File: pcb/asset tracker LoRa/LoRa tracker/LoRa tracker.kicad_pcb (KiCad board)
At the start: 2 copper layers, 100 x 100 mm, 57 parts, among them CON1 jtag, CON2 jtag, J1 Screw_Terminal_01x02, J2 Screw_Terminal_01x02, Q1 BSS138, U1 INA219BxDCN, U2 R-783.3-1.0, U3 LIS3DH, U4 G3VM-61HR2(TR05), U5 DS28CM00R-A00+T, U6 nRF52810-QFxx, U7 ATSAMD21, Y1 326MhZ

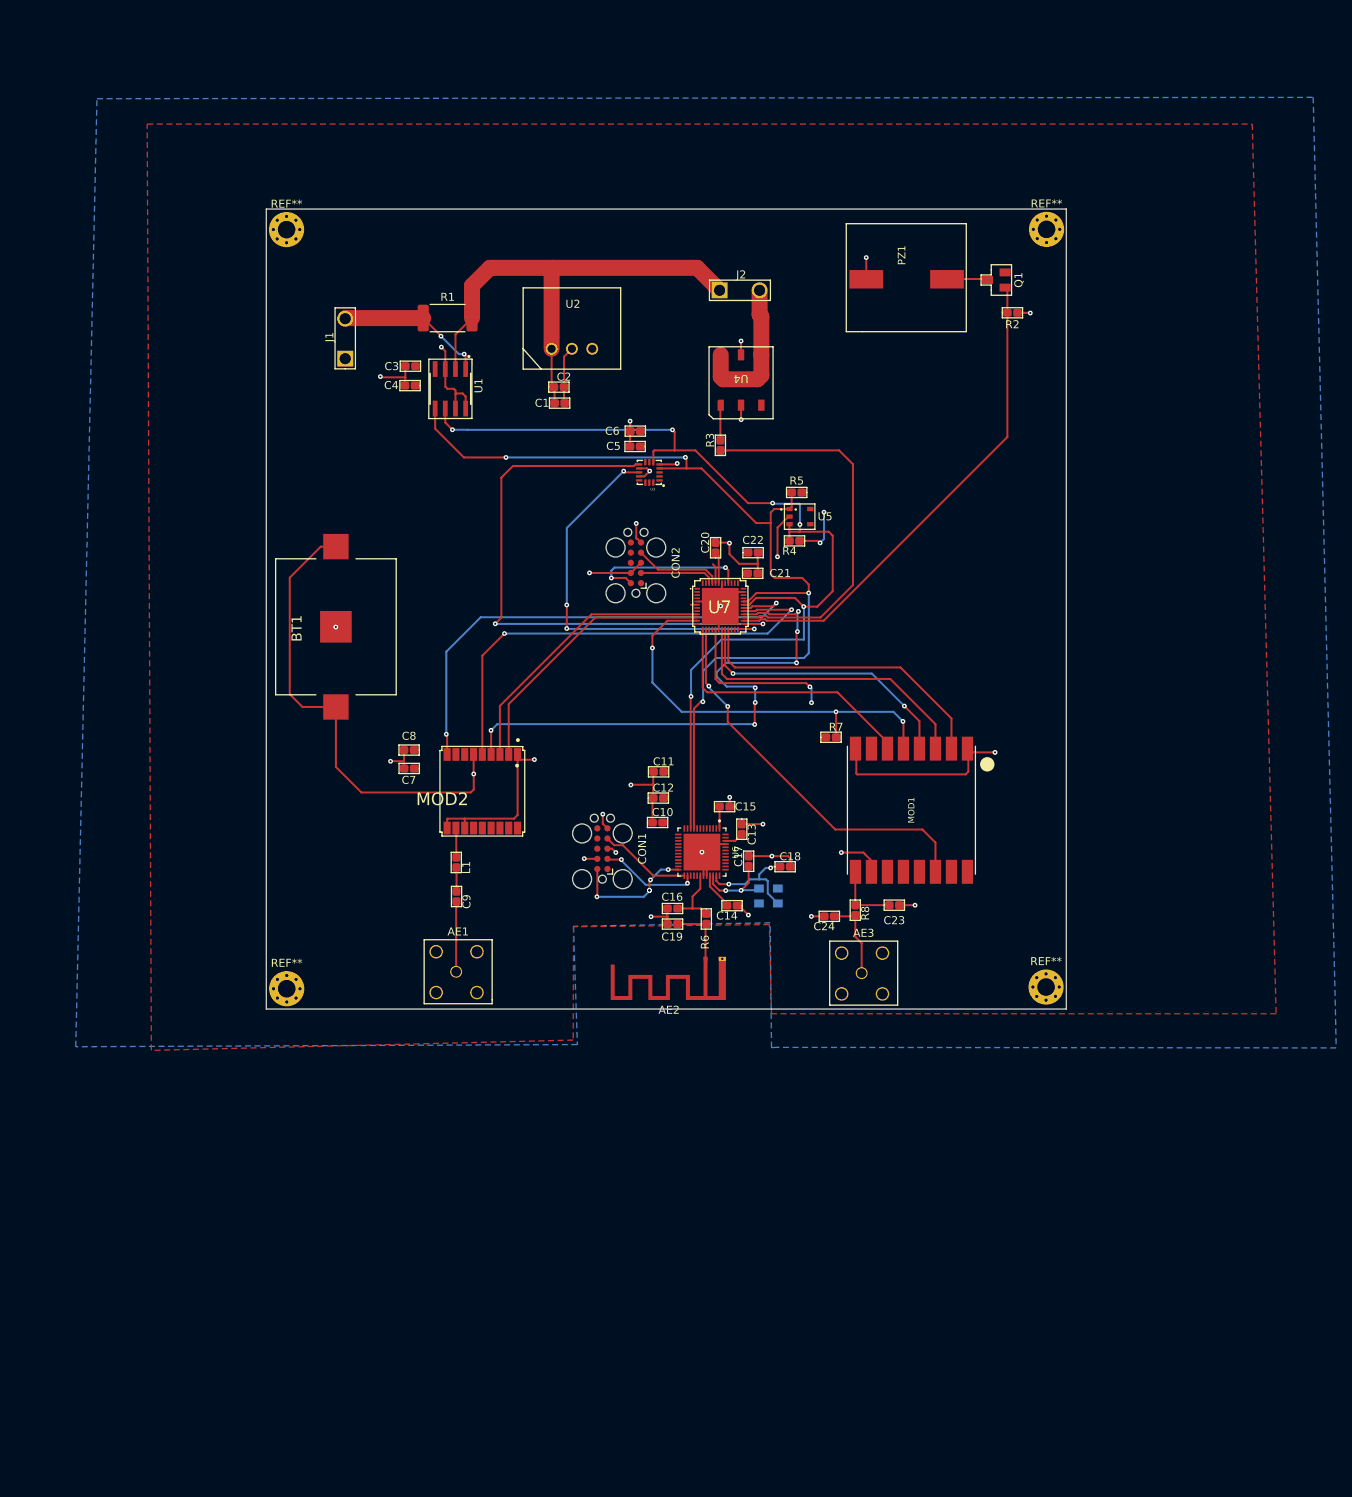
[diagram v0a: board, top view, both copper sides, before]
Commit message: pcb kastje
pcb in kastje getekend
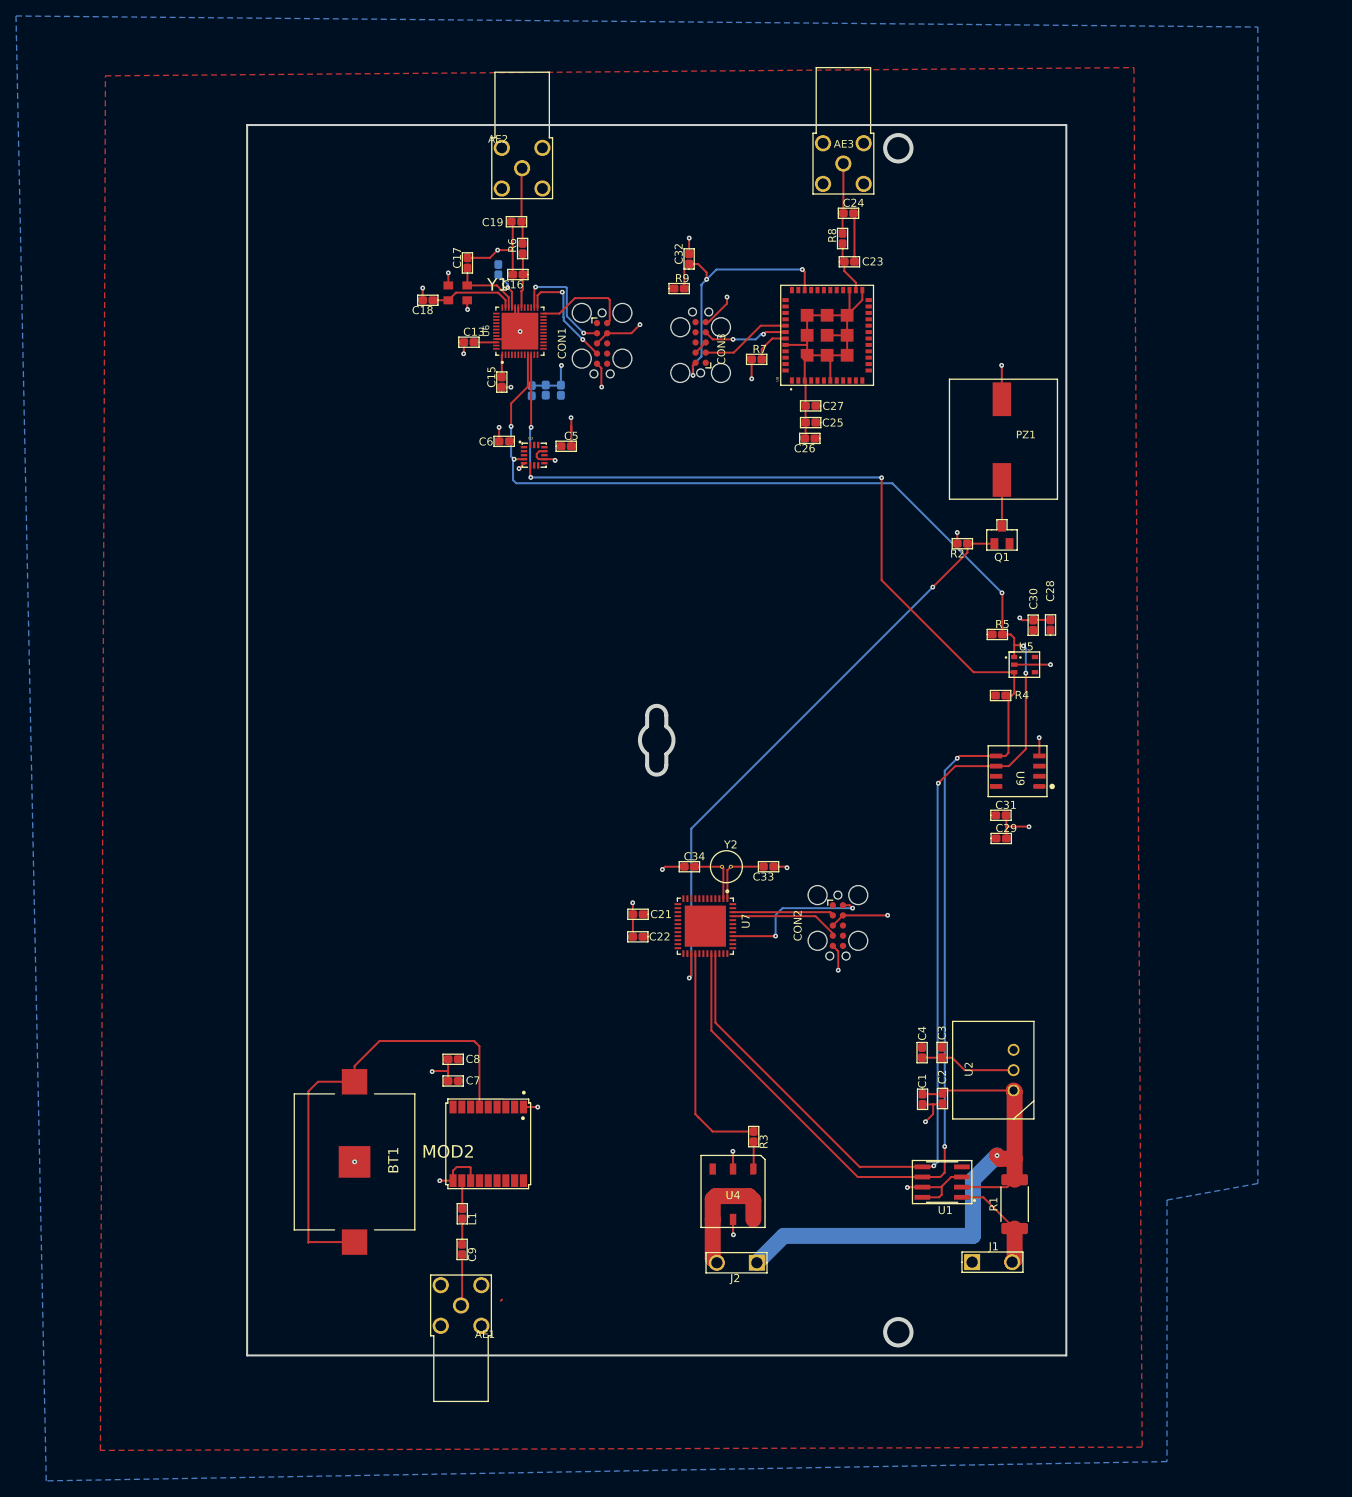
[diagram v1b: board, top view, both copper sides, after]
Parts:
- removed C20: 10uF, vanalles:0603
- removed MOD1: rfm95, Module:RFM69HW
- removed REF** (x4): MountingHole_2.2mm_M2_Pad_Via, vanalles:MountingHole_2.2mm_M2_Pad_Via
- added C25: 10uF, vanalles:0603, F.Cu at (130.2, 64.6)
- added C26: 1uF, vanalles:0603, F.Cu at (130.1, 66.5)
- added C27: 0.1uF, vanalles:0603, F.Cu at (130.2, 62.5)
- added C28: 100nF, vanalles:0603, F.Cu at (160.2, 89.8)
- added C29: 10uF, vanalles:0603, F.Cu at (154.1, 116.5)
- added C30: 100nF, vanalles:0603, F.Cu at (158.0, 89.9)
- added C31: 10uF, vanalles:0603, F.Cu at (154.0, 113.6)
- added C32: 100nF, vanalles:0603, F.Cu at (115.0, 44.1)
- added C33: 20pF, vanalles:0603, F.Cu at (125.0, 120.1)
- added C34: 20pF, vanalles:0603, F.Cu at (115.1, 120.1)
- added CON3: jtag, connectors_user:Tag-Connect_TC2050-IDC-FP_2x05_P1.27mm_Vertical, F.Cu at (116.5, 54.5)
- added R9: 10K, vanalles:0603RL, F.Cu at (113.8, 47.8)
- added U8: murattaLora, Module:XCVR_CMWX1ZZABZ-078, F.Cu at (132.3, 53.6)
- added U9: ATECC608B, halfgeleiders:soic p1.27 lengt 5.40, F.Cu at (158.8, 110.0)
- added Y2: Crystal, vanalles:crystal tht, F.Cu at (119.2, 120.1)
- AE1, AE3: footprint connectors_user:sma_right angeld -> connectors_user:sma juist
- AE2: value Antenna -> Antenna_Shield; footprint vanalles:Texas_SWRA117D_2.4GHz_Right -> connectors_user:sma juist
- C10, C11, C12, C14: moved to B.Cu
- R7: footprint vanalles:0603 -> vanalles:0603RL
- U7: value ATSAMD21 -> ATSAMD21G18A-M; footprint halfgeleiders:QFN49P40_600X600X90L40X20T460N -> halfgeleiders:QFN50P700X700X90-49N
- Y1: moved to F.Cu
- moved J1 141.0 mm to (153.0, 169.5), turned to 0 degrees
- moved R1 131.5 mm to (155.7, 162.2), turned to 90 degrees
- moved J2 121.5 mm to (121.0, 169.6), turned to 180 degrees
- moved U1 116.7 mm to (146.7, 159.5), turned to 180 degrees
- moved C3 108.5 mm to (146.7, 143.3), turned to -90 degrees
- moved U4 108.1 mm to (120.5, 164.2), turned to 0 degrees
- moved U2 105.7 mm to (155.6, 145.5), turned to 90 degrees
- moved AE2 105.6 mm to (94.2, 28.5)
- moved AE3 105.4 mm to (134.3, 28.0), turned to 180 degrees
- moved C4 105.1 mm to (144.2, 143.3), turned to -90 degrees
- moved C2 101.0 mm to (146.7, 149.0), turned to -90 degrees
- moved C1 98.1 mm to (144.2, 149.1), turned to -90 degrees
- moved C19 89.9 mm to (93.5, 39.4)
- moved C24 87.9 mm to (135.0, 38.4), turned to 0 degrees
- moved R6 86.9 mm to (94.2, 42.8), turned to 90 degrees
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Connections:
- net /LoRa_RFM/ANT_RFM renamed /LoRa_RFM/ANT
- AE2 pad 1: Net-(AE2-Pad1) -> (no net)
- AE2 pad 2: (no net) -> GND
- AE3 pad 1: unconnected-(AE3-Pad1) -> Net-(AE3-Pad1)
- C19 pad 1: Net-(AE2-Pad1) -> (no net)
- C24 pad 1: Net-(C24-Pad1) -> Net-(AE3-Pad1)
- R6 pad 2: Net-(AE2-Pad1) -> (no net)
- R7 pad 1: +3V3 -> GND
- R7 pad 2: /CS -> Net-(R7-Pad2)
- R8 pad 2: Net-(C24-Pad1) -> Net-(AE3-Pad1)
- U7 pad 1: unconnected-(U7-Pad1) -> Net-(C33-Pad2)
- U7 pad 10: /TX -> /RX
- U7 pad 11: /CS -> /TX
- U7 pad 13: /RESET -> unconnected-(U7-Pad13)
- U7 pad 14: /IRQ -> unconnected-(U7-Pad14)
- U7 pad 19: /MOSI -> unconnected-(U7-Pad19)
- U7 pad 2: unconnected-(U7-Pad2) -> Net-(C34-Pad2)
- U7 pad 20: /SCK -> unconnected-(U7-Pad20)
- U7 pad 21: /MISO -> /MOSI
- U7 pad 22: unconnected-(U7-Pad22) -> /SCK
- U7 pad 23: unconnected-(U7-Pad23) -> /CS
- U7 pad 24: /INT1 -> /MISO
- U7 pad 25: /INT2 -> /INT1
- U7 pad 26: /BUZZER -> /INT2
- U7 pad 27: /SSR -> /BUZZER
- U7 pad 28: /PPS -> /SSR
- U7 pad 29: /WAKE -> /PPS
- U7 pad 30: /RESET_GPS -> /WAKE
- U7 pad 31: /SDA -> /RESET_GPS
- U7 pad 32: /SCL -> /SDA
- U7 pad 33: unconnected-(U7-Pad33) -> /SCL
- U7 pad 39: unconnected-(U7-Pad39) -> /RESET
- U7 pad 43: Net-(C20-Pad1) -> +3V3
- U7 pad 49: GND -> unconnected-(U7-Pad49)
- U7 pad 9: /RX -> unconnected-(U7-Pad9)
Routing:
- net /SCL: track 122.8 -> 212.7 mm, vias 4 -> 7
- net /SDA: track 126.2 -> 211.8 mm, vias 6 -> 5
- net /INT2: track 72.4 -> 0.00 mm, vias 2 -> 0
- net /PPS: track 71.0 -> 0.00 mm, vias 7 -> 0
- net /RESET_GPS: track 61.0 -> 0.00 mm, vias 2 -> 0
- net /WAKE: track 59.5 -> 0.00 mm, vias 2 -> 0
- net /CS: track 52.2 -> 0.00 mm, vias 3 -> 0
- net /INT1: track 50.2 -> 0.00 mm, vias 4 -> 0
- net /IRQ: track 48.6 -> 0.00 mm, vias 2 -> 0
- net /MISO: track 38.6 -> 0.00 mm
- net /MOSI: track 37.9 -> 0.00 mm
- net /RX: track 35.5 -> 0.00 mm
- net /SCK: track 35.1 -> 0.00 mm, vias 2 -> 0
- net /TX: track 34.3 -> 0.00 mm
- net +3V3: track 30.4 -> 6.17 mm, vias 4 -> 1
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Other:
- board size 100 x 100 mm -> 102.4 x 153.8 mm
